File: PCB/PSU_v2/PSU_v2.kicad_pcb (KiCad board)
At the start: 2 copper layers, 42.5 x 38.7 mm, 19 parts, among them J1 CONN_01X05, Q1 MPSA55, Q2 IRF630, U1 MC34063

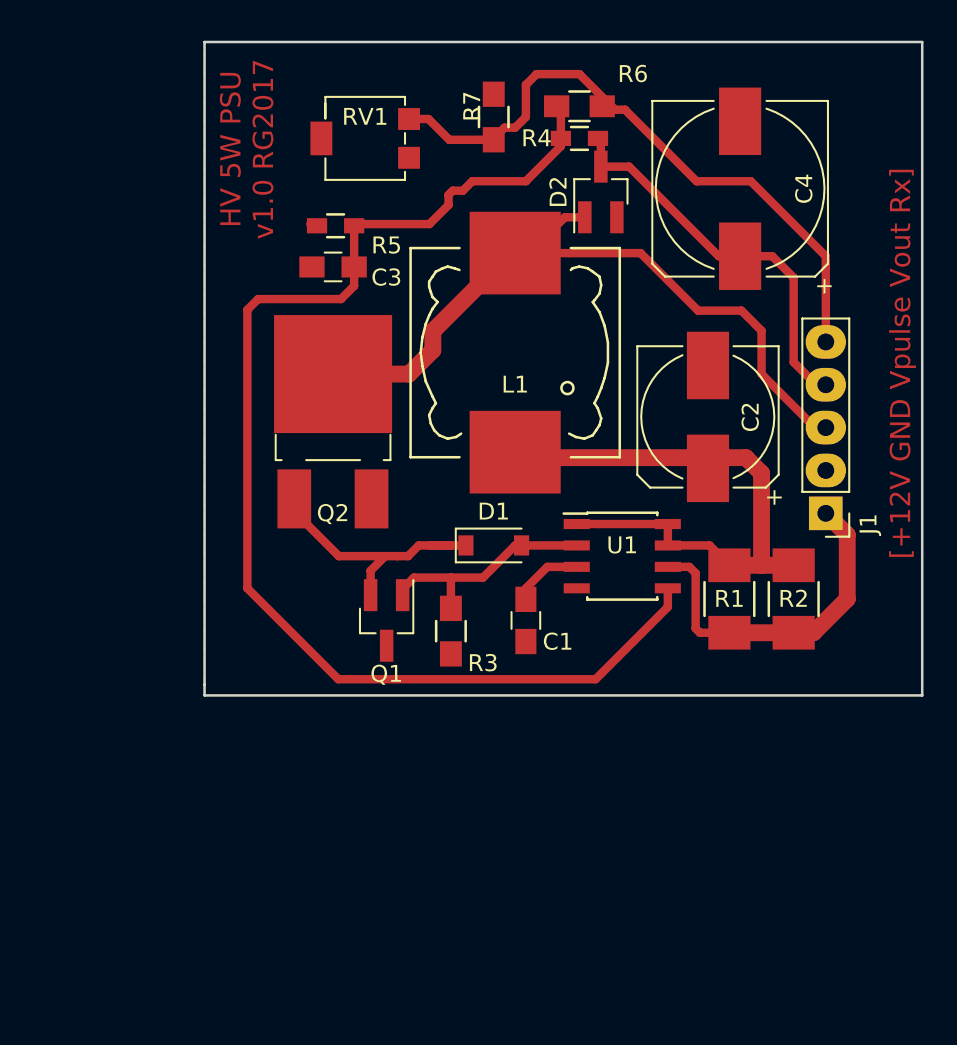
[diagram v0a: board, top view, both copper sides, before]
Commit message: PCB for HV PSU v2 prototype
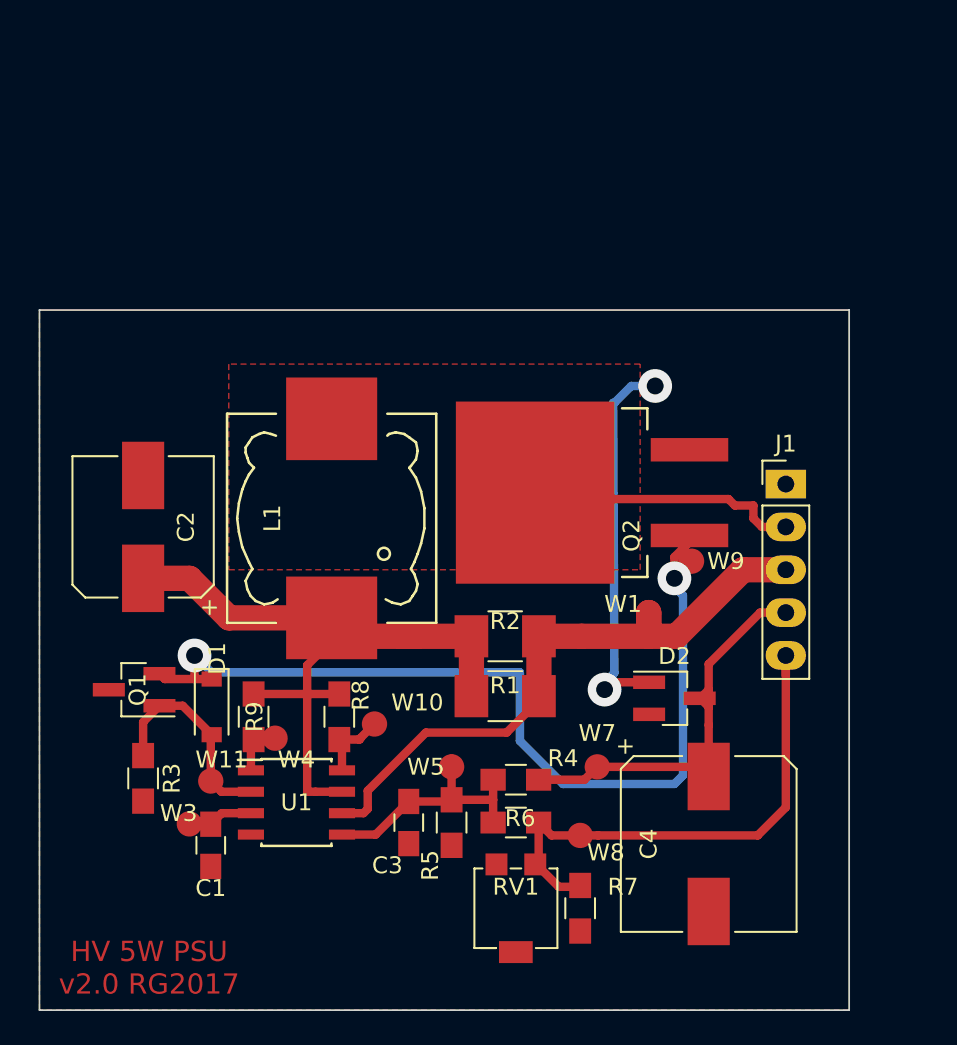
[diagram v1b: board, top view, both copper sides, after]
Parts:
- added R8: 0R, Resistors_SMD:R_0805_HandSoldering, F.Cu at (129.3, 94.6)
- added R9: 0R, Resistors_SMD:R_0805_HandSoldering, F.Cu at (124.2, 94.6)
- added W1: TEST_1P, Measurement_Points:Measurement_Point_Round-SMD-Pad_Small, F.Cu at (147.6, 88.4)
- added W10: TEST_1P, Measurement_Points:Measurement_Point_Round-SMD-Pad_Small, F.Cu at (131.4, 95.0)
- added W11: TEST_1P, Measurement_Points:Measurement_Point_Round-SMD-Pad_Small, F.Cu at (121.7, 98.4)
- added W3: TEST_1P, Measurement_Points:Measurement_Point_Round-SMD-Pad_Small, F.Cu at (120.4, 101.0)
- added W4: TEST_1P, Measurement_Points:Measurement_Point_Round-SMD-Pad_Small, F.Cu at (125.5, 95.9)
- added W5: TEST_1P, Measurement_Points:Measurement_Point_Round-SMD-Pad_Small, F.Cu at (135.9, 97.6)
- added W7: TEST_1P, Measurement_Points:Measurement_Point_Round-SMD-Pad_Small, F.Cu at (144.6, 97.6)
- added W8: TEST_1P, Measurement_Points:Measurement_Point_Round-SMD-Pad_Small, F.Cu at (143.6, 101.6)
- added W9: TEST_1P, Measurement_Points:Measurement_Point_Round-SMD-Pad_Small, F.Cu at (150.2, 85.4)
- Q2: footprint TO_SOT_Packages_SMD:TO-252-2Lead -> nixie_fp:TO-263-2Lead
- R4: value 475k -> 330k; footprint Resistors_SMD:R_0603_HandSoldering -> Resistors_SMD:R_0805_HandSoldering
- R5: value 13.7k -> 3.3k; footprint Resistors_SMD:R_0603_HandSoldering -> Resistors_SMD:R_0805_HandSoldering
- R6: value 4.02k -> 5.6k
- moved R7 47.2 mm to (143.6, 106.0), turned to 90 degrees
- moved RV1 46.5 mm to (139.7, 106.0), turned to 90 degrees
- moved R6 42.6 mm to (139.7, 100.9)
- moved C4 38.9 mm to (151.2, 102.2), turned to 270 degrees
- moved R4 38.2 mm to (139.7, 98.3)
- moved R5 36.0 mm to (135.9, 100.9), turned to 270 degrees
- moved C2 34.1 mm to (117.6, 83.4)
- moved C3 33.2 mm to (133.4, 100.9), turned to 270 degrees
- moved D2 30.3 mm to (149.1, 93.5), turned to 0 degrees
- moved U1 24.2 mm to (126.7, 99.7)
- moved C1 22.9 mm to (121.7, 102.2)
- moved Q2 21.4 mm to (150.0, 81.3), turned to 180 degrees
- moved R3 20.2 mm to (117.6, 98.3)
- moved D1 19.3 mm to (121.7, 94.0), turned to 270 degrees
- moved R2 17.2 mm to (139.1, 89.8), turned to 0 degrees
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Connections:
- net Net-(C1-Pad1) renamed /MC_C_t
- net Net-(C3-Pad1) renamed /MC_CMP
- net Net-(D1-Pad1) renamed /MOSFET_G
- net Net-(D1-Pad2) renamed /MC_Es
- J1 pad 1: +12V -> GND
- J1 pad 2: GND -> /Vpulse
- J1 pad 3: /Vpulse -> +12V
- RV1 pad 1: /Rx -> Net-(RV1-Pad1)
- RV1 pad 3: Net-(RV1-Pad3) -> /Rx
- U1 pad 1: Net-(C2-Pad1) -> /MC_Cs
- U1 pad 8: Net-(C2-Pad1) -> /MC_Cd
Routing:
- net /MC_CMP: track 74.6 -> 14.8 mm
- net /MOSFET_G: track 16.8 -> 55.6 mm, vias 0 -> 2
- net +12V: track 20.7 -> 38.1 mm
- net Net-(C2-Pad1): track 35.3 -> 44.3 mm
- net /Rx: track 37.5 -> 31.7 mm
- net /MC_Cd: track 0.00 -> 4.49 mm
- net /MC_Cs: track 0.00 -> 3.19 mm
- net /Vout: track 23.2 -> 24.6 mm
- net /MC_Es: track 13.6 -> 12.6 mm
- net /Vpulse: track 43.6 -> 43.8 mm, vias 0 -> 2
- added copper zone on F.Cu, net /Vpulse
- removed copper zone on F.Cu, net (none)
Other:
- board size 42.5 x 38.7 mm -> 48 x 41.5 mm
- net class Default: via_dia 1 -> 2; via_drill 0.5 -> 1
- net class HV: clearance 1 -> 1.5; via_dia 1 -> 2; via_drill 0.5 -> 1
- net class Power: trace_width 1 -> 1.5; via_dia 1 -> 2; via_drill 0.5 -> 1
- rule pad_to_mask_clearance: 0.2 -> 0
- rule trace_min: 0.5 -> 0.2
- rule via_min_drill: 0.5 -> 0.3
- rule via_min_size: 1 -> 0.4
- board text added: "HV 5W PSU v2.0 RG2017"
- board text removed: "HV 5W PSU v1.0 RG2017"
- board text removed: "[+12V GND Vpulse Vout Rx]"
